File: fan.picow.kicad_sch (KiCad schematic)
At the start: 41 parts, among them U1 PicoW

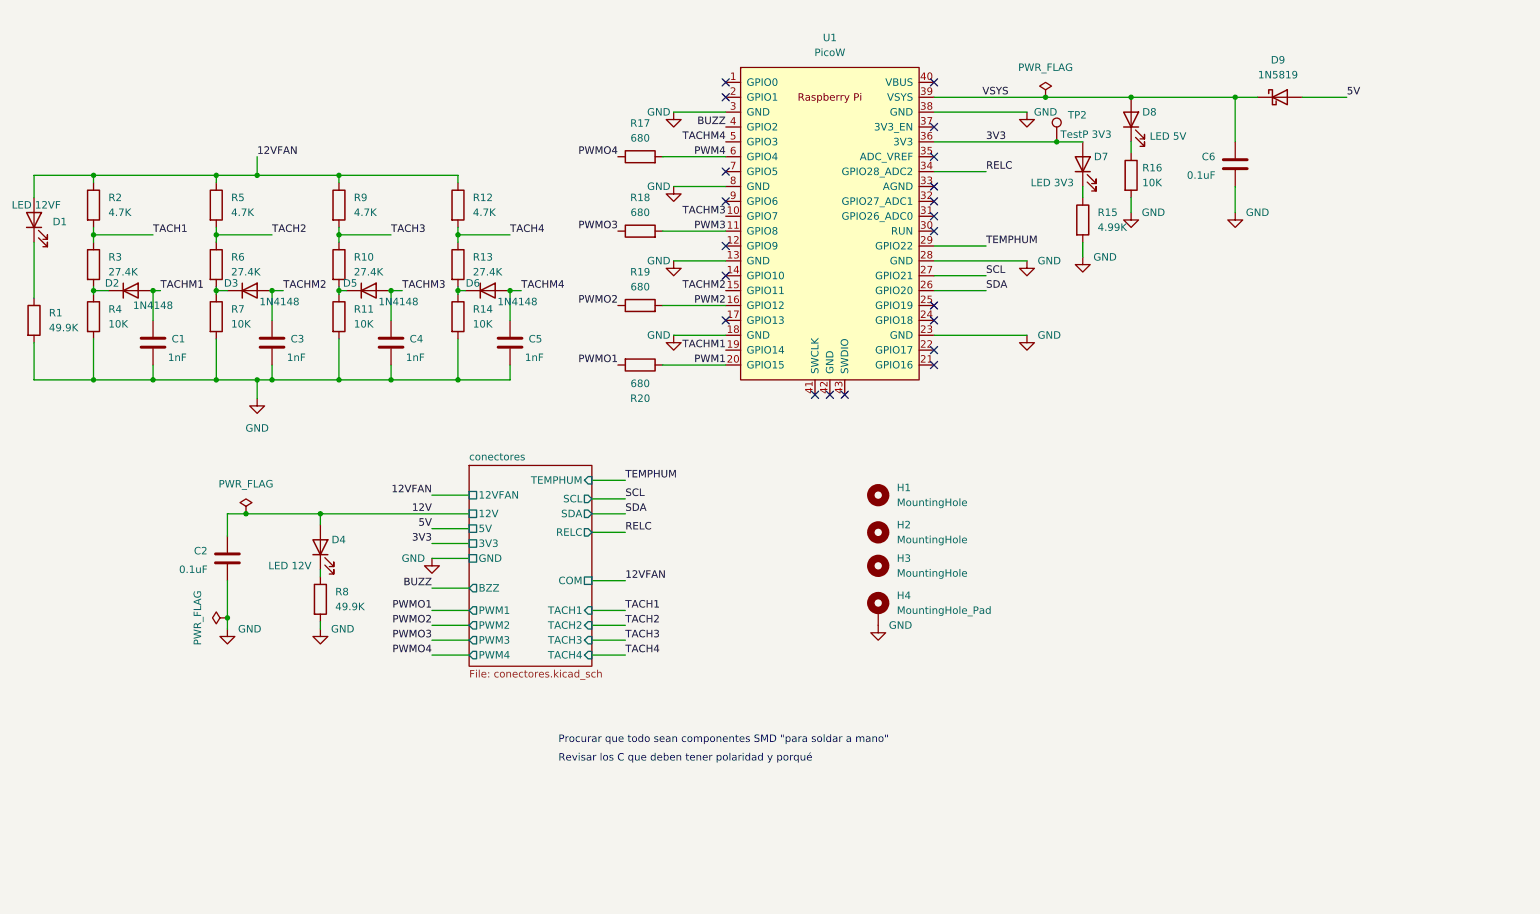
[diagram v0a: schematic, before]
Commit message: pop stashed changes
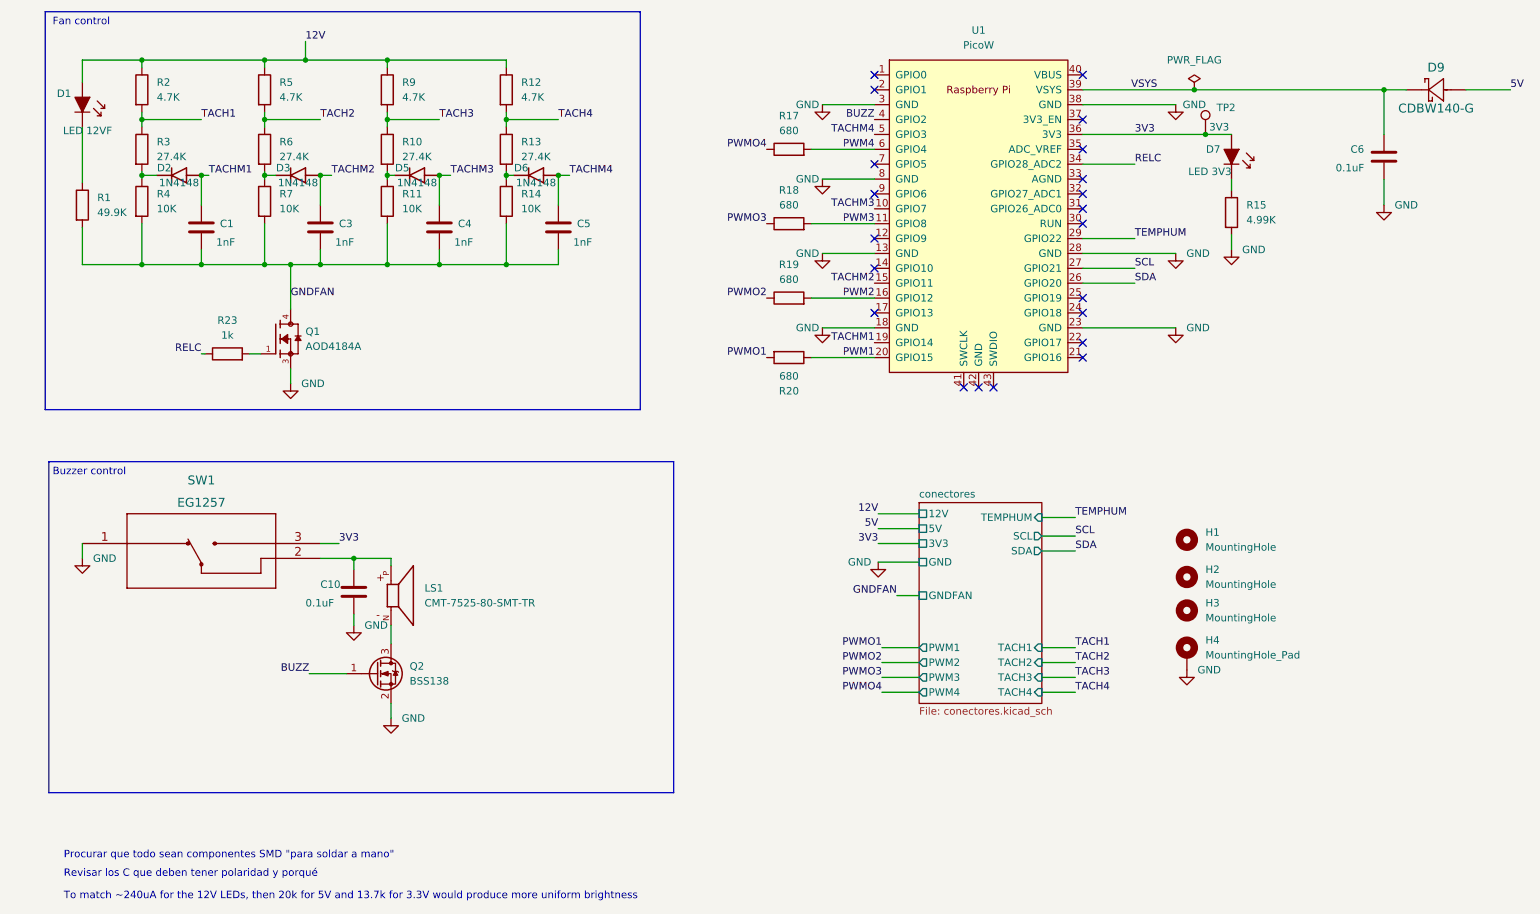
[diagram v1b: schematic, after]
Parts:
- removed C2: 0.1uF, Capacitor_SMD:C_0603_1608Metric_Pad1.08x0.95mm_HandSolder, symbol Device:C
- removed D4: LED 12V, LED_SMD:LED_0805_2012Metric_Pad1.15x1.40mm_HandSolder, symbol Device:LED
- removed D8: LED 5V, LED_SMD:LED_0805_2012Metric_Pad1.15x1.40mm_HandSolder, symbol Device:LED
- removed D9: 1N5819, Diode_SMD:D_SMA_Handsoldering, symbol Diode:1N5819
- removed R16: 10K, Resistor_SMD:R_0603_1608Metric_Pad0.98x0.95mm_HandSolder, symbol Device:R
- removed R8: 49.9K, Resistor_SMD:R_0603_1608Metric_Pad0.98x0.95mm_HandSolder, symbol Device:R
- added C10: 0.1uF, Capacitor_SMD:C_0603_1608Metric_Pad1.08x0.95mm_HandSolder, symbol Device:C
- added D9: CDBW140-G, Diode_SMD:D_SOD-123F, symbol CDBW140-G:CDBW140-G
- added LS1: CMT-7525-80-SMT-TR, footprints descargados:XDCR_CMT-7525-80-SMT-TR, symbol CMT-7525-80-SMT-TR:CMT-7525-80-SMT-TR
- added Q1: AOD4184A, footprints descargados:DPAK228P994X240-4N, symbol AOD4184A:AOD4184A
- added Q2: BSS138, Package_TO_SOT_SMD:SOT-23, symbol Transistor_FET:BSS138
- added R23: 1k, Resistor_SMD:R_0603_1608Metric_Pad0.98x0.95mm_HandSolder, symbol Device:R
- added SW1: EG1257, footprints descargados:EG1257, symbol EG1257:EG1257
- D1, D7: footprint LED_SMD:LED_0805_2012Metric_Pad1.15x1.40mm_HandSolder -> digikey-footprints:0805; symbol Device:LED -> dk_LED-Indication-Discrete:LG_R971-KN-1; Category (none) -> Optoelectronics; DK_Datasheet_Link (none) -> https://dammedia.osram.info/media/resource/hires/osram-dam-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; DK_Detail_Page (none) -> /product-detail/en/osram-opto-semiconductors-inc/LG-R971-KN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; Digi-Key_PN (none) -> 475-1410-1-ND; Family (none) -> LED Indication - Discrete; MPN (none) -> LG R971-KN-1; Manufacturer (none) -> OSRAM Opto Semiconductors Inc.; Status (none) -> Active
- D2, D3, D5, D6: footprint Diode_SMD:D_SMA_Handsoldering -> Diode_SMD:D_SOD-123; symbol Diode:1N4148 -> 1N4148W:1N4148W
- TP2: value TestP 3V3 -> 3V3
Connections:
- net 12V: now also D1.1, R12.1, R2.1, R5.1, R9.1
- net 3V3: now also D7.1, SW1.3; no longer D7.2 (A)
- net 5V: now also D9.2
- net BUZZ: now also Q2.1 (G)
- net GND: now also C10.2, Q1.3, Q2.2 (S), SW1.1; no longer C1.2, C3.2, C4.2, C5.2, R1.2, R11.2, R14.2, R4.2, R7.2
- net RELC: now also R23.1
- net TACHM1: now also D2.1; no longer D2.2 (A)
- net TACHM2: now also D3.1; no longer D3.2 (A)
- net TACHM3: now also D5.1; no longer D5.2 (A)
- net TACHM4: now also D6.1; no longer D6.2 (A)
- net VSYS: now also D9.1
- net at R15.1: now also D7.2; no longer D7.1 (K)
- net at R10.2, R11.1: now also D5.2; no longer D5.1 (K)
- net at R3.2, R4.1: now also D2.2; no longer D2.1 (K)
- net at R6.2, R7.1: now also D3.2; no longer D3.1 (K)
- net at R13.2, R14.1: now also D6.2; no longer D6.1 (K)
- net at R1.1: now also D1.2; no longer D1.1 (K)
- removed net 12VFAN: D1.2 (A), R12.1, R2.1, R5.1, R9.1
- new net: LS1.N, Q2.3 (D)
- new net: C10.1, LS1.P, SW1.2
- new net: Q1.1, R23.2
- new net GNDFAN: C1.2, C3.2, C4.2, C5.2, Q1.4, R1.2, R11.2, R14.2, R4.2, R7.2
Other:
- sheet conectores ports: added GNDFAN; removed 12VFAN, BZZ, COM, RELC
- note added: "Buzzer control"
- note added: "Fan control"
- note added: "To match ~240uA for the 12V LEDs, then 20k for 5V and 13.7k for 3.3V would produce more uniform brightness"
- moved on the sheet: C1, C3, C4, C5, C6, H1, H2, H3, H4, R1, R10, R11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
